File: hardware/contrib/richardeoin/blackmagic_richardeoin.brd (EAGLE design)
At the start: 27 parts, among them IC1 STM32F_48PIN, IC2 TXS0108, Q1 IRLML5103, Y1 8MHz

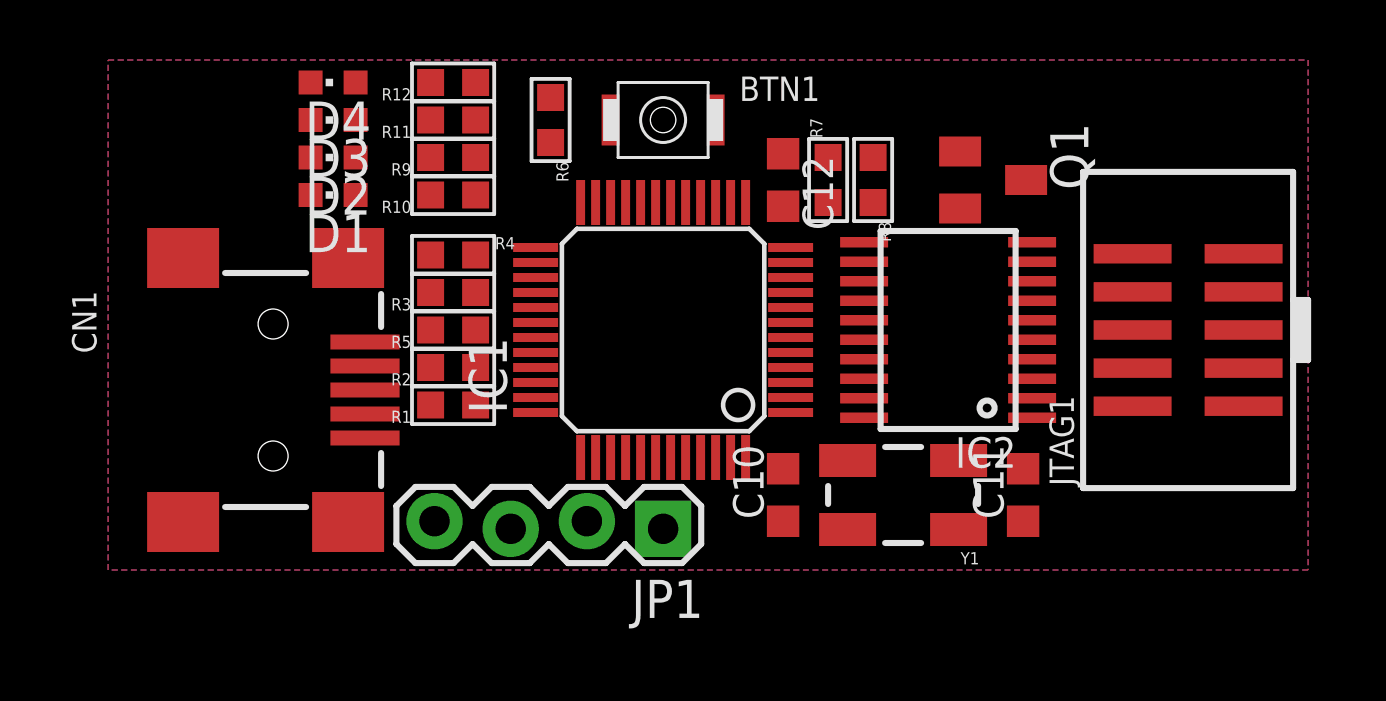
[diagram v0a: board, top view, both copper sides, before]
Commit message: Schematic provisionally complete
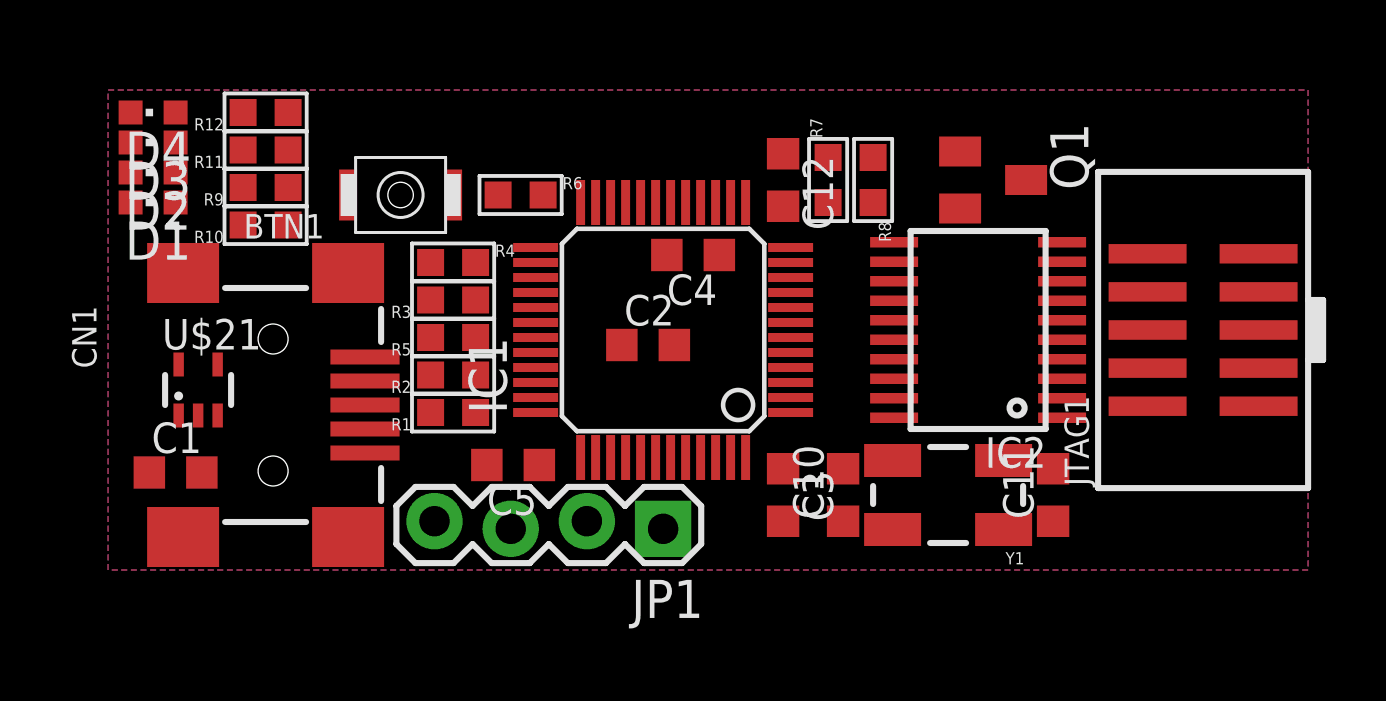
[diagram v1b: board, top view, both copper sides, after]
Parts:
- added C1, C2: 1µF, resistor:C0603K
- added C3, C4, C5: 100nF, resistor:C0603K
- added U$21: TLV70033DCK, tlv700:SC70-5L
- moved BTN1 9.10 mm to (9.75, 12.5), turned to 180 degrees
- moved R10 6.33 mm to (5.25, 11.5)
- moved R11 6.33 mm to (5.25, 14.0)
- moved R12 6.33 mm to (5.25, 15.2)
- moved R9 6.33 mm to (5.25, 12.8)
- moved D4 6.08 mm to (1.50, 15.2)
- moved D3 6.05 mm to (1.50, 14.2)
- moved D2 6.02 mm to (1.50, 13.2)
- moved D1 6.01 mm to (1.50, 12.2)
- moved R6 2.69 mm to (13.8, 12.5), turned to 0 degrees
- moved C10 2.00 mm to (24.5, 2.50)
- moved Y1 1.50 mm to (28.0, 2.50)
- moved C11 1.00 mm to (31.5, 2.50)
- moved IC2 1.00 mm to (29.0, 8.00)
- moved CN1 0.50 mm to (4.50, 5.50)
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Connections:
- net 3.3V: now also C2.1, C3.1, C4.1, C5.1, U$21.5
- net 5.0V: now also C1.1, U$21.1, U$21.3
- net GND: now also C1.2, C2.2, C3.2, C4.2, C5.2, U$21.2
